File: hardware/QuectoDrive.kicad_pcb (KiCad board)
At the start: 2 copper layers, 15.2 x 12.1 mm, 27 parts, among them U1 SPX3819M5-L-1-8, U2 ATtiny1616-M, U3 DRV8837, U4 DRV8837

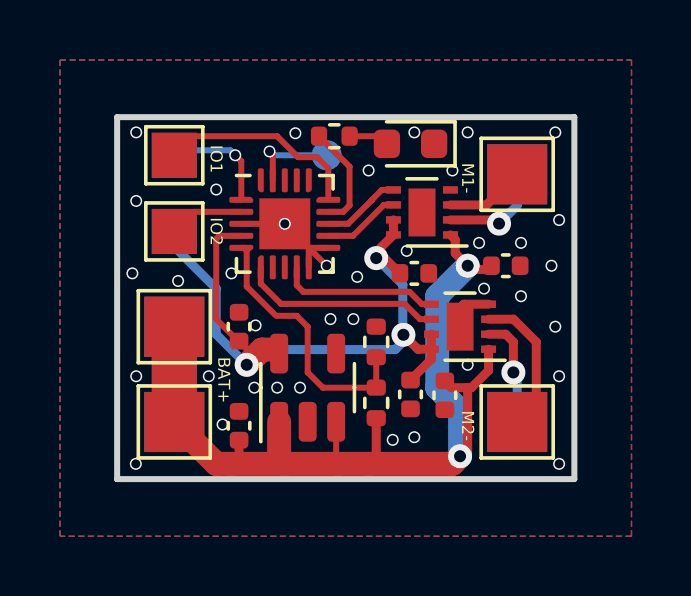
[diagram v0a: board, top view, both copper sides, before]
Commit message: Board Rev 2
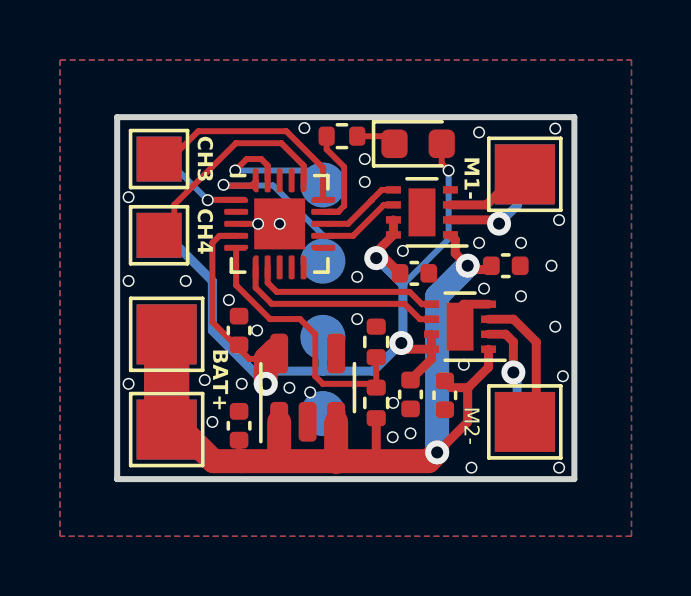
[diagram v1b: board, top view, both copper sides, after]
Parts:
- added TP13: PROG, TestPoint:TestPoint_Pad_D1.5mm, B.Cu at (97.0, 90.5)
- added TP14: PROG, TestPoint:TestPoint_Pad_D1.5mm, B.Cu at (97.0, 85.4)
- added TP7: PROG, TestPoint:TestPoint_Pad_D1.5mm, B.Cu at (97.0, 88.0)
- TP5: footprint TestPoint:TestPoint_Pad_D1.0mm -> TestPoint:TestPoint_Pad_D1.5mm
- moved TP5 1.00 mm to (97.0, 82.9)
- moved TP10 0.52 mm to (91.6, 82.0)
- moved TP6 0.52 mm to (91.6, 84.6)
- moved TP8 0.52 mm to (91.6, 84.6)
- moved TP9 0.52 mm to (91.6, 82.0)
- moved TP1 0.36 mm to (91.8, 87.9)
- moved TP3 0.36 mm to (91.8, 87.9)
- moved TP2 0.36 mm to (91.8, 91.1)
- moved TP4 0.36 mm to (91.8, 91.1)
- moved D1 0.25 mm to (100.2, 81.5), turned to 0 degrees
- moved TP11 0.25 mm to (103.8, 90.8)
- moved TP12 0.25 mm to (103.8, 90.8)
- moved TP15 0.25 mm to (103.8, 82.5)
- moved TP16 0.25 mm to (103.8, 82.5)
- moved R1 0.25 mm to (97.7, 81.3)
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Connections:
- C1 pad 1: +3V3 -> +3.3V
- C5 pad 1: +3V3 -> +3.3V
- C6 pad 1: +3V3 -> +3.3V
- D1 pad 1: GND -> Net-(D1-K)
- D1 pad 2: Net-(D1-Pad2) -> +3.3V
- R1 pad 2: Net-(D1-Pad2) -> Net-(D1-K)
- TP8 pad 1: +3V3 -> +3.3V
- U1 pad 5: +3V3 -> +3.3V
- U2 pad 10: GND -> unconnected-(U2-PB4-Pad10)
- U2 pad 11: GND -> unconnected-(U2-PB3-Pad11)
- U2 pad 16: unconnected-(U2-Pad16) -> /IO_2
- U2 pad 2: /IO_2 -> unconnected-(U2-PA3-Pad2)
- U2 pad 20: unconnected-(U2-Pad20) -> /DEBUG_TX
- U2 pad 4: +3V3 -> +3.3V
- U2 pad 7: unconnected-(U2-Pad7) -> /MOT_2B
- U2 pad 9: /MOT_2B -> unconnected-(U2-PB5-Pad9)
- U3 pad 7: +3V3 -> +3.3V
- U3 pad 8: +3V3 -> +3.3V
- U4 pad 7: +3V3 -> +3.3V
- U4 pad 8: +3V3 -> +3.3V
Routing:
- net +3.3V: track 0.00 -> 34.6 mm, vias 0 -> 4
- net +3V3: track 26.3 -> 0.00 mm, vias 3 -> 0
- net /DEBUG_TX: track 0.00 -> 5.95 mm, vias 0 -> 1
- net GND: track 10.7 -> 5.74 mm, vias 38 -> 35
- net /IO_2: track 2.50 -> 6.85 mm
- net +BATT: track 32.8 -> 30.0 mm
- net /UDPI: track 2.97 -> 4.90 mm
- net Net-(D1-Pad2): track 1.35 -> 0.00 mm
- net Net-(D1-K): track 0.00 -> 1.35 mm
- net /MOT_2B: track 5.35 -> 6.27 mm
- net /IBUS: track 3.74 -> 3.08 mm
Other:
- board text added: "2023"
- board text added: "CH3"
- board text added: "CH4"
- board text removed: "22/01/2023"
- board text removed: "IO1"
- board text removed: "IO2"
- board text removed: "JLCJLCJLCJLC"
- board text removed: "PROG"
